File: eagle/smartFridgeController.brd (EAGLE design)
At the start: 35.9 x 45.7 mm, 12 parts

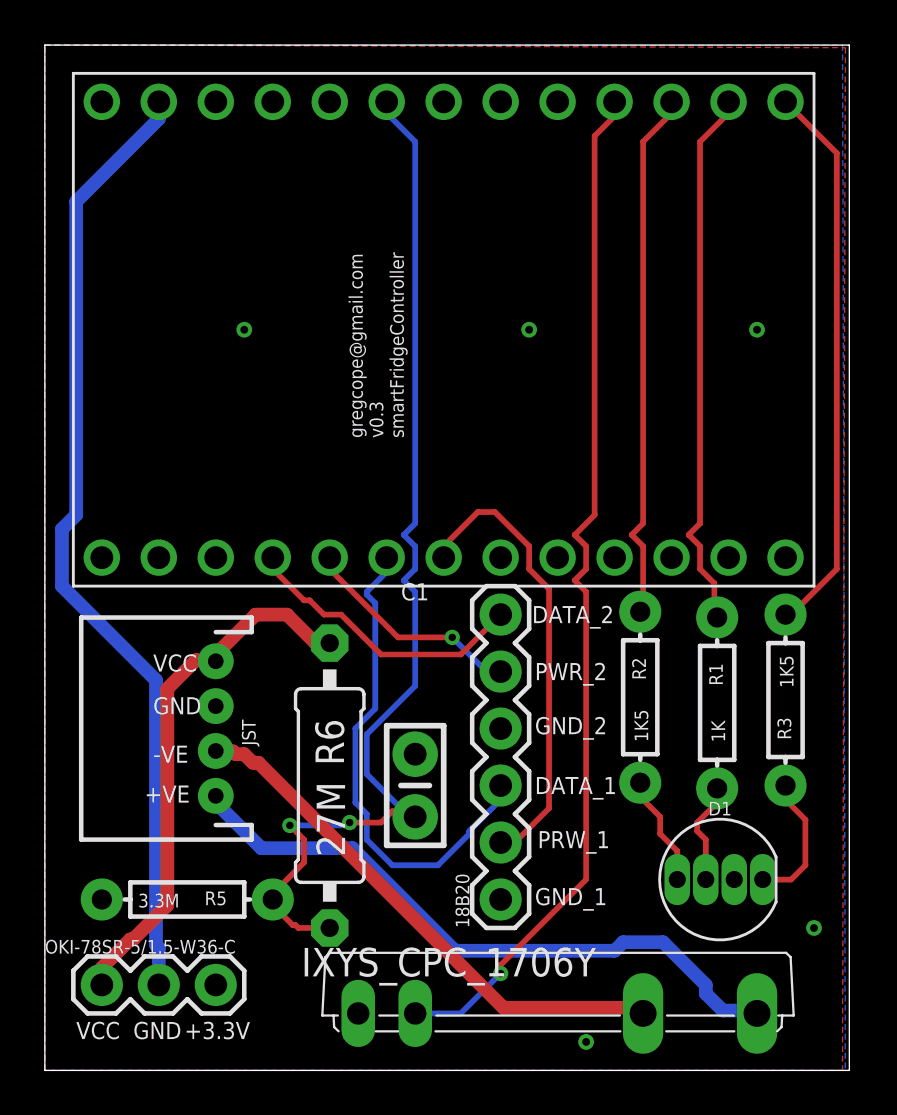
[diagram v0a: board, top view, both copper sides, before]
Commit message: New layout, 0.3
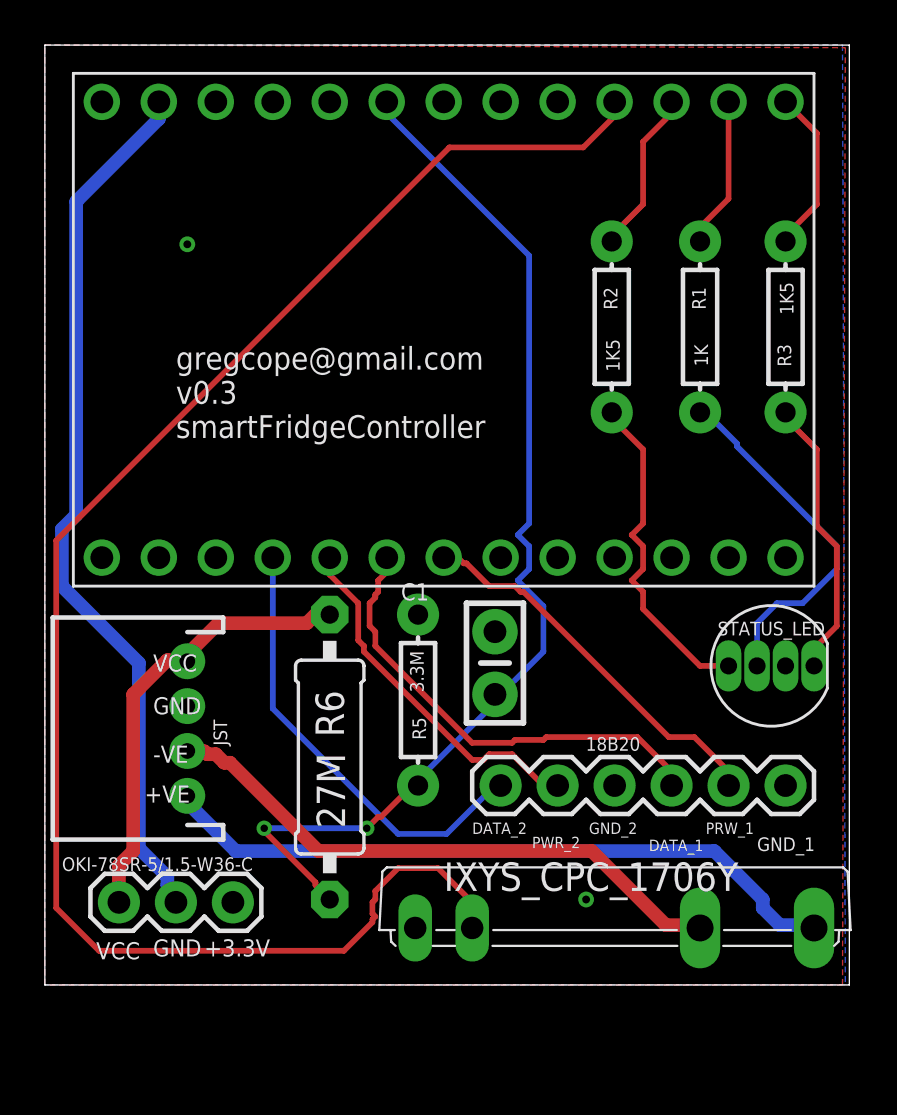
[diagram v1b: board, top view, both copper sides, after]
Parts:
- removed D1: CLEAR, SparkFun-LED:LED-RGB-THRU
- added STATUS_LED: CLEAR, SparkFun-LED:LED-RGB-THRU
- JST: value (none) -> 18B20
- moved R1 16.8 mm to (27.9, 33.1)
- moved R3 16.6 mm to (31.8, 33.1)
- moved R2 16.6 mm to (24.0, 33.1)
- moved 18B20 13.7 mm to (31.8, 12.7), turned to 180 degrees
- moved R5 13.6 mm to (15.4, 16.5), turned to 270 degrees
- moved C1 6.52 mm to (18.8, 18.2)
- moved IXYS_CPC_1706Y 4.58 mm to (24.1, 6.35)
- moved OKI-78SR-5/1.5-W36-C 3.76 mm to (2.03, 7.49)
- moved R6 1.27 mm to (11.4, 14.0)
- moved JST 1.27 mm to (5.08, 15.2)
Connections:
- net GND: now also STATUS_LED.2
- net N$1: now also STATUS_LED.1; no longer D1.1
- net N$2: now also STATUS_LED.4; no longer D1.4
- net N$3: now also STATUS_LED.3; no longer D1.3
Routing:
- net D17_RELAY_PIN: track 46.4 -> 73.2 mm, vias 1 -> 0
- net D14_LED_RED_PIN: track 24.9 -> 7.38 mm
- net D15_LED_GREEN_PIN: track 24.2 -> 6.75 mm
- net D16_LED_BLUE_PIN: track 23.7 -> 7.33 mm
- net N$3: track 4.59 -> 16.1 mm
- net N$2: track 5.00 -> 15.0 mm
- net D4_DS2_DATA: track 13.0 -> 20.1 mm
- net N$1: track 6.09 -> 12.7 mm
- net D5_DS2_PWR: track 10.0 -> 16.1 mm, vias 1 -> 0
- net VCC: track 23.8 -> 20.0 mm
- net VIN: track 42.9 -> 39.6 mm
- net D7_DS1_PWR: track 20.4 -> 17.3 mm
- net -VE: track 23.9 -> 26.1 mm
- net +VE: track 28.9 -> 30.8 mm
- net D6_DS1_DATA: track 22.0 -> 20.7 mm
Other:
- board size 35.9 x 45.7 mm -> 35.9 x 41.9 mm
